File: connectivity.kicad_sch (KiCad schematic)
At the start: 55 parts, among them CN1 GPS_Port, Con2 DS1023-1X2SF11, J1 USB_C_Receptacle, J10 DS1023-1X8SF11, J11 DS1023-1X5SF11, J12 DS1023-1X5SF11, J13 DS1023-1X5SF11, J14 DS1023-1X5SF11, J15 DS1023-1X5SF11, J16 DS1023-1X5SF11, J17 DS1023-1X5SF11, J2 JST_GH_SM06B-GHS-TB, J3 JST_GH_SM06B-GHS-TB, J4 JST_GH_SM06B-GHS-TB, J5 JST_GH_SM06B-GHS-TB, J6 DS1023-1X11S21, J7 DS1023-1X11S21, J8 DS1023-1X6SF11, J9 DS1023-1X11S21, U3 SN65HVD232, con1 DS1023-1X3SF11

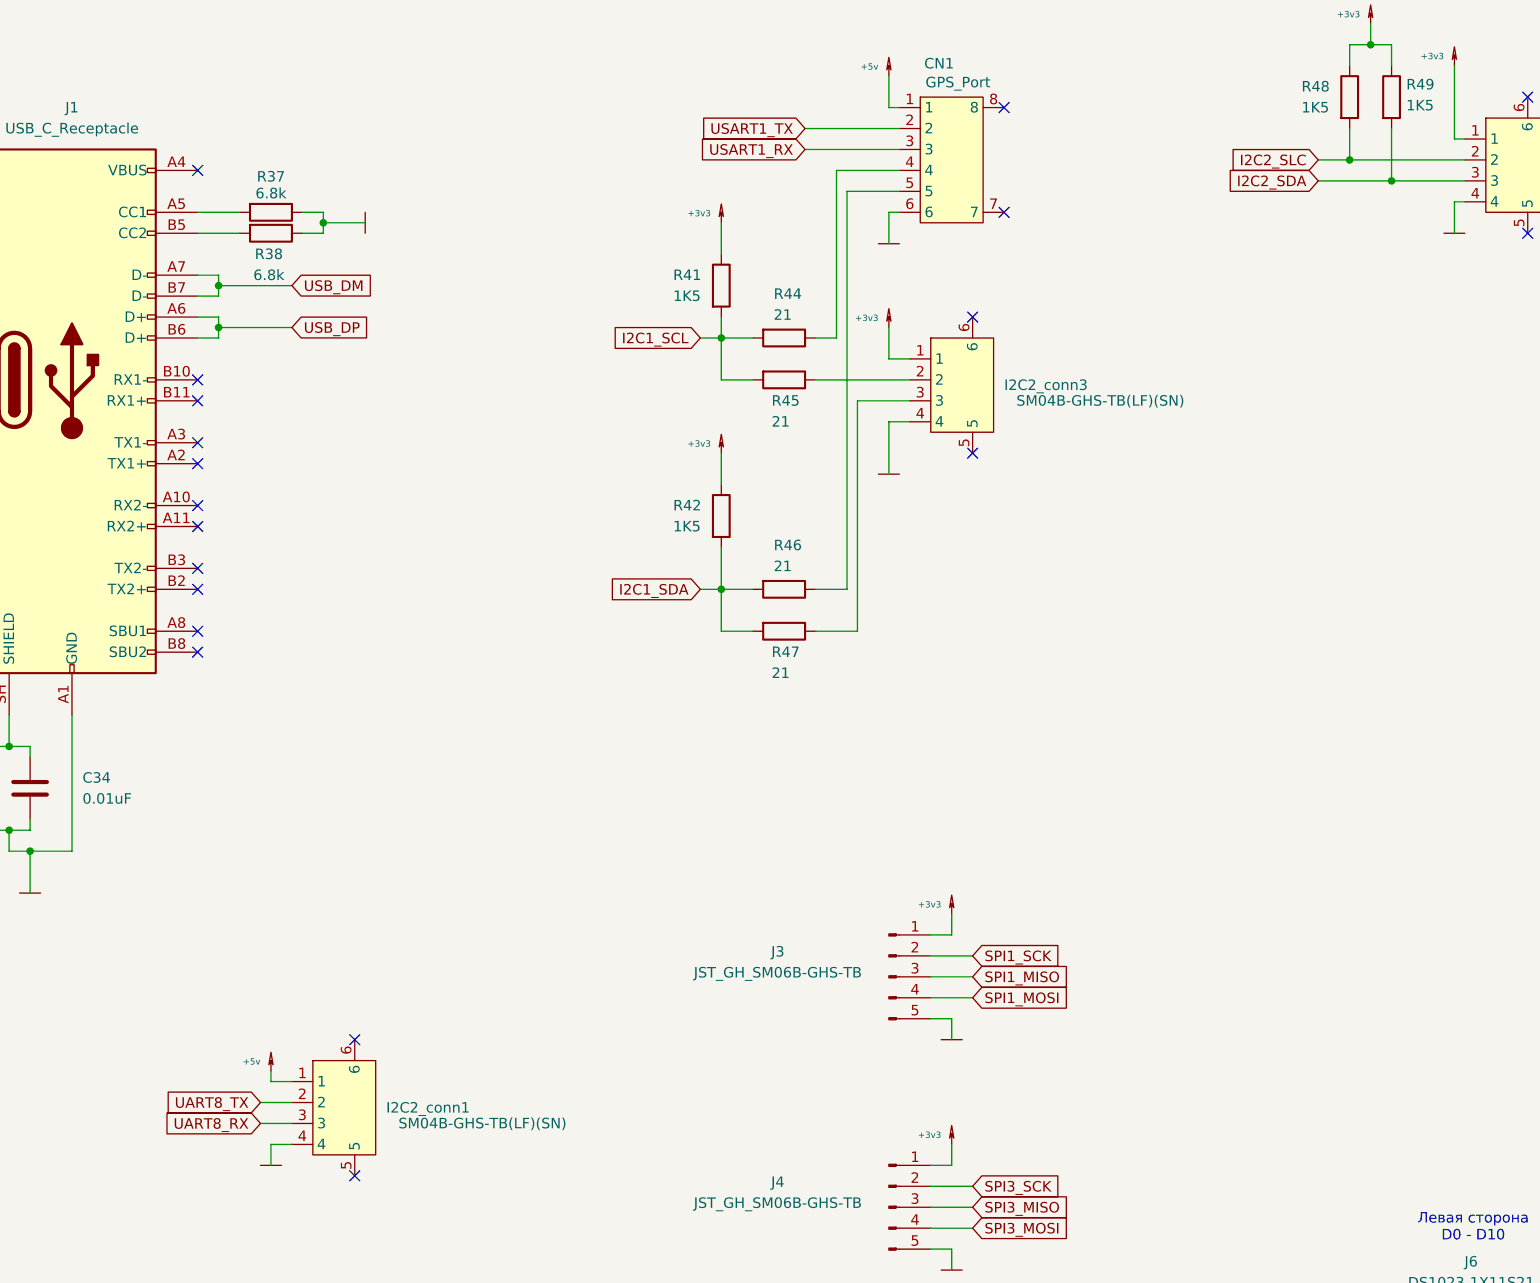
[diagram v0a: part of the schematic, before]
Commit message: Дорожки
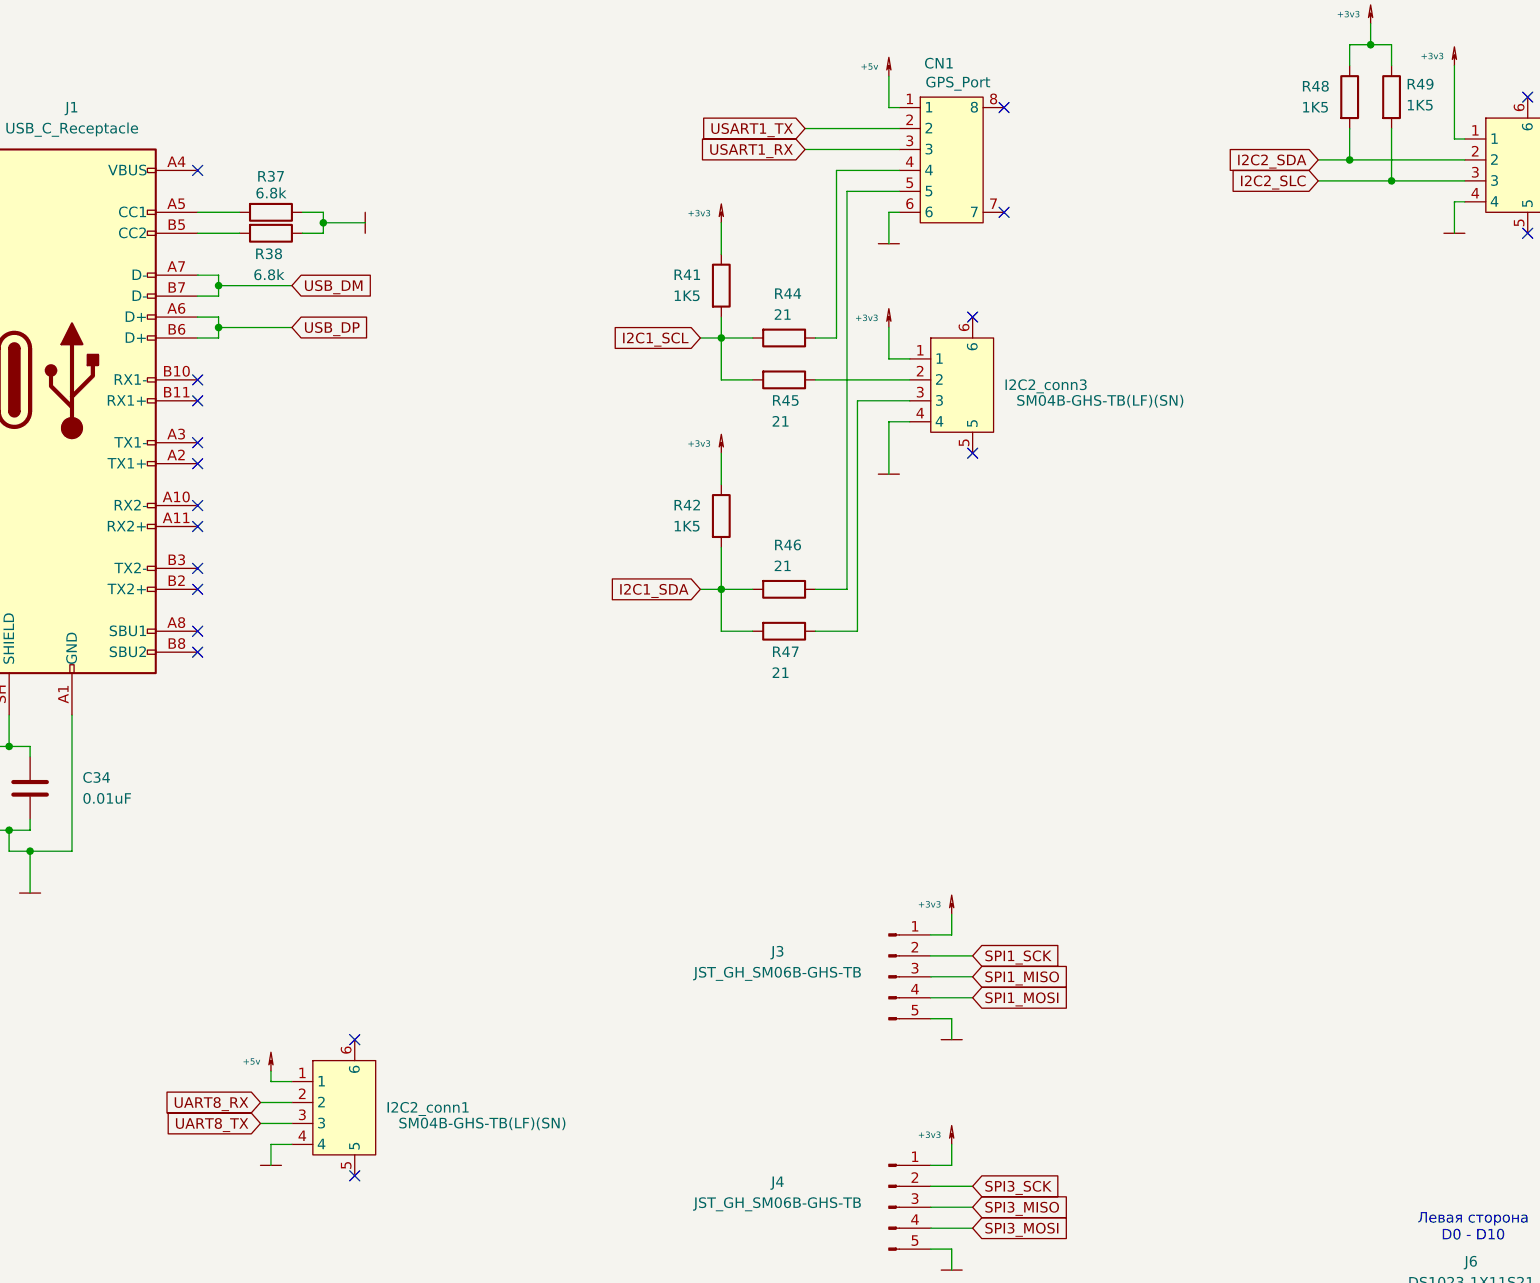
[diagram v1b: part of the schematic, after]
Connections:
- net I2C2_SDA: now also I2C2_conn4.2, R48.2; no longer I2C2_conn4.3, R49.2
- net I2C2_SLC: now also I2C2_conn4.3, R49.2; no longer I2C2_conn4.2, R48.2
- net UART8_RX: now also I2C2_conn1.2; no longer I2C2_conn1.3
- net UART8_TX: now also I2C2_conn1.3; no longer I2C2_conn1.2
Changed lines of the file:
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@@
 	)
 	(junction
+		(at 190.5 45.72)
+		(diameter 0)
+		(color 0 0 0 0)
+	)
+	(junction
 		(at 53.34 60.96)
 		(diameter 0)
@@
 	)
 	(junction
-		(at 190.5 45.72)
+		(at 195.58 48.26)
 		(diameter 0)
 		(color 0 0 0 0)
@@
 	)
 	(junction
-		(at 195.58 48.26)
-		(diameter 0)
-		(color 0 0 0 0)
-	)
-	(junction
 		(at 114.3 67.31)
 		(diameter 0)
@@
 	(wire
 		(pts
+			(xy 58.42 162.56) (xy 62.23 162.56)
+		)
+		(stroke
+			(width 0)
+			(type default)
+		)
+	)
+	(wire
+		(pts
 			(xy 261.62 156.21) (xy 265.43 156.21)
 		)
@@
 	(wire
 		(pts
-			(xy 195.58 48.26) (xy 186.69 48.26)
-		)
-		(stroke
-			(width 0)
-			(type default)
-		)
-	)
-	(wire
-		(pts
 			(xy 269.24 93.98) (xy 273.05 93.98)
 		)
@@
 	(wire
 		(pts
+			(xy 58.42 160.02) (xy 62.23 160.02)
+		)
+		(stroke
+			(width 0)
+			(type default)
+		)
+	)
+	(wire
+		(pts
 			(xy 219.71 170.18) (xy 223.52 170.18)
 		)
@@
 	(wire
 		(pts
-			(xy 58.42 160.02) (xy 62.23 160.02)
-		)
-		(stroke
-			(width 0)
-			(type default)
-		)
-	)
-	(wire
-		(pts
 			(xy 134.62 52.07) (xy 134.62 55.88)
 		)
@@
 	(wire
 		(pts
+			(xy 186.69 48.26) (xy 195.58 48.26)
+		)
+		(stroke
+			(width 0)
+			(type default)
+		)
+	)
+	(wire
+		(pts
+			(xy 186.69 45.72) (xy 190.5 45.72)
+		)
+		(stroke
+			(width 0)
+			(type default)
+		)
+	)
+	(wire
+		(pts
 			(xy 219.71 193.04) (xy 223.52 193.04)
 		)
@@
 	(wire
 		(pts
-			(xy 190.5 45.72) (xy 186.69 45.72)
-		)
-		(stroke
-			(width 0)
-			(type default)
-		)
-	)
-	(wire
-		(pts
 			(xy 50.8 59.69) (xy 53.34 59.69)
 		)
@@
 	(wire
 		(pts
-			(xy 58.42 162.56) (xy 62.23 162.56)
-		)
-		(stroke
-			(width 0)
-			(type default)
-		)
-	)
-	(wire
-		(pts
 			(xy 275.59 26.67) (xy 283.21 26.67)
 		)
@@
 	(global_label "UART8_RX"
 		(shape input)
-		(at 58.42 162.56 180)
+		(at 58.42 160.02 180)
 		(effects
 			(font
@@
 		)
 		(property "Intersheetrefs" "${INTERSHEET_REFS}"
-			(at 58.42 162.56 0)
+			(at 58.42 160.02 0)
 			(hide yes)
 			(show_name no)
@@
 	(global_label "I2C2_SLC"
 		(shape input)
-		(at 186.69 45.72 180)
+		(at 186.69 48.26 180)
 		(fields_autoplaced yes)
 		(effects
@@
 		)
 		(property "Intersheetrefs" "${INTERSHEET_REFS}"
-			(at 174.9358 45.72 0)
+			(at 174.9358 48.26 0)
 			(hide yes)
 			(show_name no)
@@
 	(global_label "UART8_TX"
 		(shape input)
-		(at 58.42 160.02 180)
+		(at 58.42 162.56 180)
 		(effects
 			(font
@@
 		)
 		(property "Intersheetrefs" "${INTERSHEET_REFS}"
-			(at 58.42 160.02 0)
+			(at 58.42 162.56 0)
 			(hide yes)
 			(show_name no)
@@
 	(global_label "I2C2_SDA"
 		(shape input)
-		(at 186.69 48.26 180)
+		(at 186.69 45.72 180)
 		(fields_autoplaced yes)
 		(effects
@@
 		)
 		(property "Intersheetrefs" "${INTERSHEET_REFS}"
-			(at 174.8753 48.26 0)
+			(at 174.8753 45.72 0)
 			(hide yes)
 			(show_name no)
